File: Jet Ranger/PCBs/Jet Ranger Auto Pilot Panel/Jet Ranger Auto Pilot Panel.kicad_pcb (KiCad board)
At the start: 2 copper layers, 75.5 x 79.5 mm, 35 parts, among them J1 AP OLED, J2 BACKLIGHT, J3 AUTOPILOT, SW1 ENC_CRS, SW10 AP_APPR, SW11 AP_FD, SW12 AP_BC, SW2 ENC_ALT, SW3 ENC_VS, SW4 ENC_IAS, SW5 ENC_HDG, SW6 AP_ENABLE, SW7 AP_HDG, SW8 AP_CRS, SW9 AP_ALT

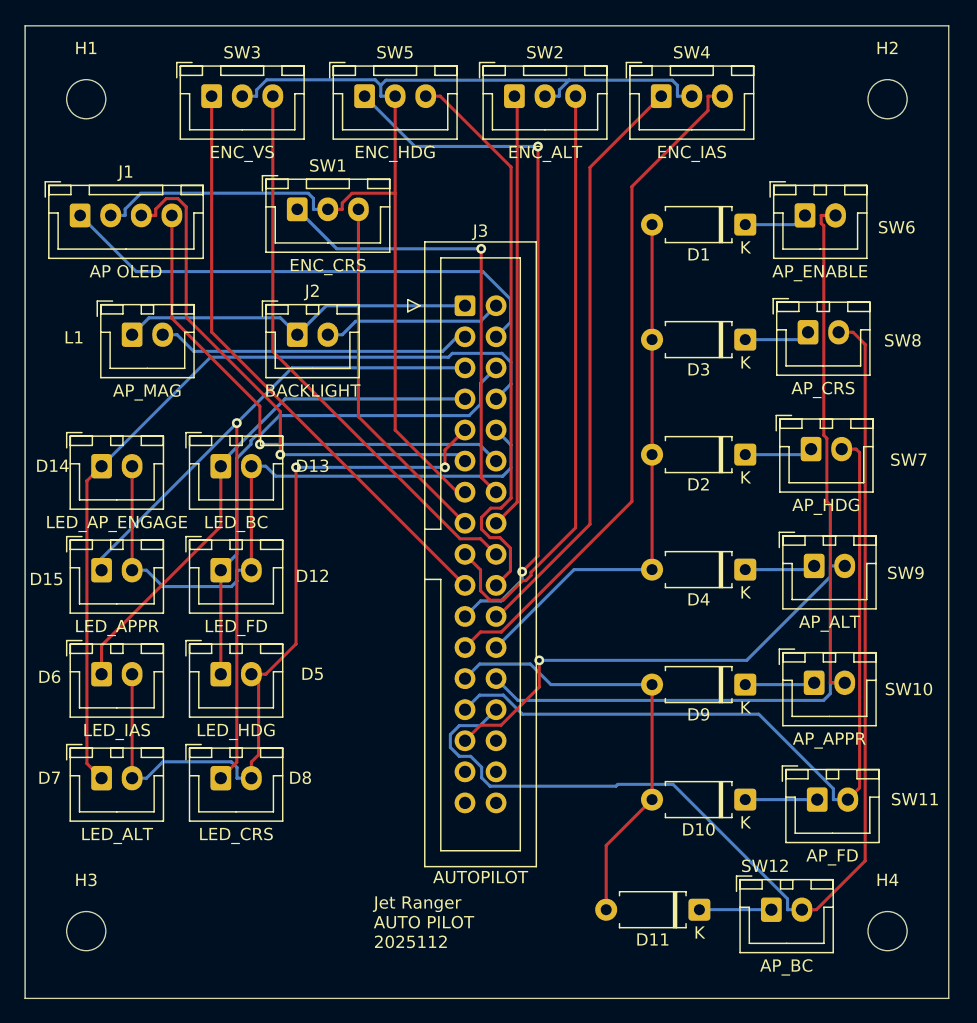
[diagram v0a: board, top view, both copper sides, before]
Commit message: Jet Ranger
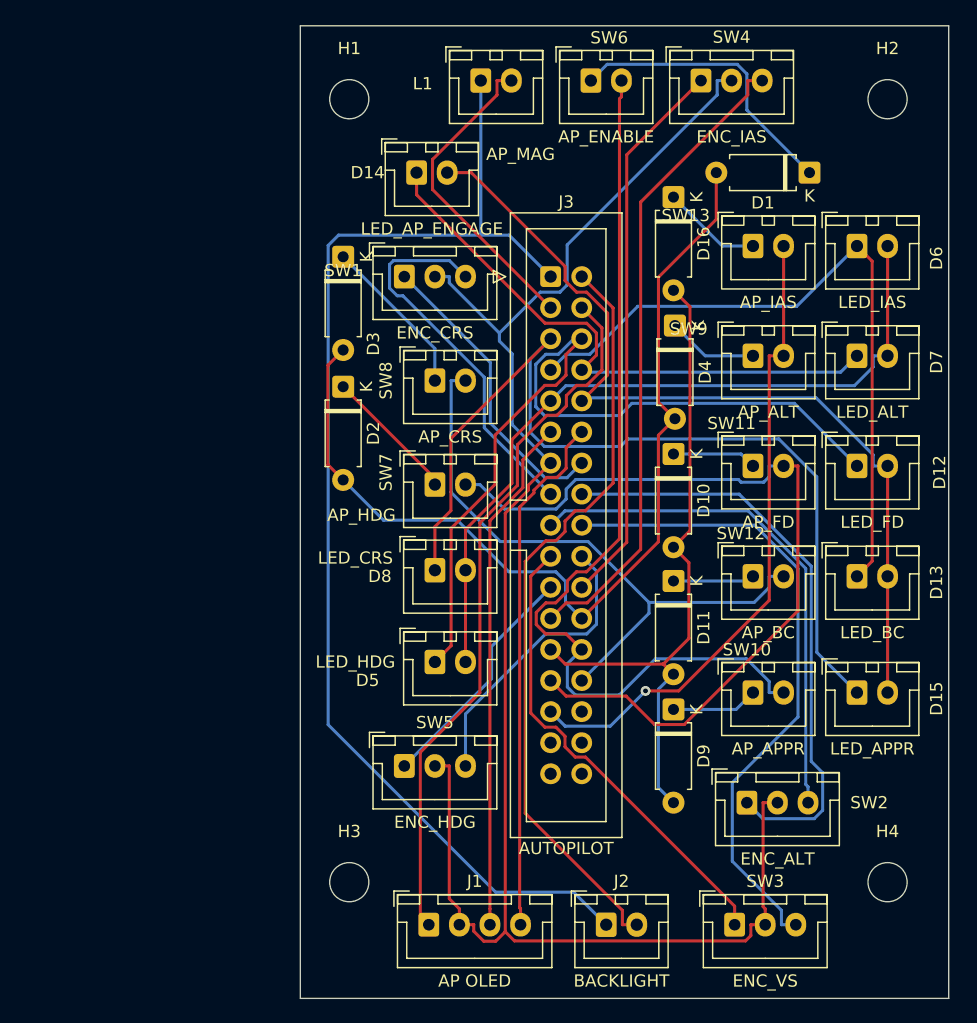
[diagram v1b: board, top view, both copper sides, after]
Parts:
- added D16: D, Diode_THT:D_A-405_P7.62mm_Horizontal, F.Cu at (142.0, 91.5)
- added SW13: AP_IAS, Connector_JST:JST_XH_B2B-XH-A_1x02_P2.50mm_Vertical, F.Cu at (148.5, 95.5)
- moved SW3 80.1 mm to (147.0, 151.0)
- moved D6 71.0 mm to (157.0, 95.5)
- moved D7 70.7 mm to (157.0, 104.5)
- moved J1 64.6 mm to (122.0, 151.0)
- moved D15 62.6 mm to (157.0, 132.0)
- moved SW2 60.8 mm to (148.0, 141.0)
- moved SW5 54.8 mm to (120.0, 138.0)
- moved J2 54.4 mm to (136.5, 151.0)
- moved D13 52.8 mm to (157.0, 122.5)
- moved D12 52.7 mm to (157.0, 113.5)
- moved L1 35.3 mm to (126.2, 82.0)
- moved D14 35.2 mm to (121.0, 89.5)
- moved D3 33.6 mm to (115.0, 96.4), turned to -90 degrees
- moved D2 33.3 mm to (115.0, 107.0), turned to -90 degrees
- moved SW7 30.9 mm to (122.5, 115.0)
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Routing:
- net /+12v-IN: track 29.3 -> 101.2 mm
- net /BACKLIGHT_PANELS: track 14.7 -> 62.4 mm
- net ROW2: track 92.6 -> 51.3 mm
- net /HDG_A: track 57.8 -> 19.6 mm, vias 2 -> 0
- net GND: track 105.2 -> 143.1 mm
- net COL1: track 43.6 -> 78.9 mm
- net /ANNODE_01: track 43.6 -> 69.1 mm
- net /HDG_B: track 47.0 -> 24.0 mm
- net /ANNODE_03: track 67.6 -> 47.8 mm
- net /CATHODE_01: track 53.8 -> 73.1 mm
- net COL2: track 36.4 -> 55.5 mm
- net Net-(D1-K): track 5.19 -> 23.8 mm
- net +3.3V: track 41.6 -> 58.5 mm
- net ROW3: track 38.8 -> 52.8 mm
- net /ANNODE_02: track 43.4 -> 57.3 mm
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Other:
- board size 75.5 x 79.5 mm -> 53 x 79.5 mm
- board text added: "Jet Ranger AUTO PILOT ${REVISION} ${ISSUE_DATE} 2025112"
- board text removed: "Jet Ranger AUTO PILOT 2025112"
